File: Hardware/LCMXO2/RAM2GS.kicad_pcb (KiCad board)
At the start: 4 copper layers, 67.3 x 48.5 mm, 64 parts, among them J1 IIgs RAM Exp., J2 JTAG, U1 LCMXO2-TG100, U10 74LVC1G04GW, U11 AP2127K-1.2TRG1, U2 W9812G6KH-6, U3 60M, U4 74AHCT245PW, U5 74LVC245APW, U6 74LVC245APW, U7 74LVC245APW, U8 AZ1117CH-3.3TRG1, U9 74LVC1G04GW

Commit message: Updated LCMXO2 board, fixed GND via
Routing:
- net GND: vias 211 -> 212
- net (no net): vias 1 -> 0
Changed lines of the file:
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@@
     (add_net "Net-(U9-Pad1)")
+  )
+  (module stdpads:R_0603 (layer F.Cu)
+    (at 75.6 119.65)
+    (tags resistor)
+    (solder_mask_margin 0.05)
+    (solder_paste_margin -0.05)
+    (attr smd)
+    (fp_text reference R8 (at 0 0) (layer F.Fab)
+      (effects (font (size 0.254 0.254) (thickness 0.0635)))
+    )
+    (fp_text value 10k (at 0 0.25) (layer F.Fab)
+      (effects (font (size 0.127 0.127) (thickness 0.03175)))
+    )
+    (fp_line (start -0.8 0.4) (end -0.8 -0.4) (layer F.Fab) (width 0.1))
+    (fp_line (start -0.8 -0.4) (end 0.8 -0.4) (layer F.Fab) (width 0.1))
+    (fp_line (start 0.8 -0.4) (end 0.8 0.4) (layer F.Fab) (width 0.1))
+    (fp_line (start 0.8 0.4) (end -0.8 0.4) (layer F.Fab) (width 0.1))
+    (fp_line (start -0.162779 -0.51) (end 0.162779 -0.51) (layer F.SilkS) (width 0.12))
+    (fp_line (start -0.162779 0.51) (end 0.162779 0.51) (layer F.SilkS) (width 0.12))
+    (fp_line (start -1.4 0.7) (end -1.4 -0.7) (layer F.CrtYd) (width 0.05))
+    (fp_line (start -1.4 -0.7) (end 1.4 -0.7) (layer F.CrtYd) (width 0.05))
+    (fp_line (start 1.4 -0.7) (end 1.4 0.7) (layer F.CrtYd) (width 0.05))
+    (fp_line (start 1.4 0.7) (end -1.4 0.7) (layer F.CrtYd) (width 0.05))
+    (fp_text user %R (at 0 0) (layer F.SilkS) hide
+      (effects (font (size 0.254 0.254) (thickness 0.0635)))
+    )
+    (pad 1 smd roundrect (at -0.8 0) (size 0.7 0.95) (layers F.Cu F.Paste F.Mask) (roundrect_rratio 0.25)
+      (net 37 +3V3))
+    (pad 2 smd roundrect (at 0.8 0) (size 0.7 0.95) (layers F.Cu F.Paste F.Mask) (roundrect_rratio 0.25)
+      (net 122 /DONE))
+    (model ${KISYS3DMOD}/Resistor_SMD.3dshapes/R_0603_1608Metric.wrl
+      (at (xyz 0 0 0))
+      (scale (xyz 1 1 1))
+      (rotate (xyz 0 0 0))
+    )
   )
   (module stdpads:TSSOP-20_4.4x6.5mm_P0.65mm (layer F.Cu)
@@
       (rotate (xyz 0 0 0))
     )
-  )
-  (module stdpads:R_0603 (layer F.Cu)
-    (at 75.6 119.65)
-    (tags resistor)
-    (solder_mask_margin 0.05)
-    (solder_paste_margin -0.05)
-    (attr smd)
-    (fp_text reference R8 (at 0 0) (layer F.Fab)
-      (effects (font (size 0.254 0.254) (thickness 0.0635)))
-    )
-    (fp_text value 10k (at 0 0.25) (layer F.Fab)
-      (effects (font (size 0.127 0.127) (thickness 0.03175)))
-    )
-    (fp_line (start 1.4 0.7) (end -1.4 0.7) (layer F.CrtYd) (width 0.05))
-    (fp_line (start 1.4 -0.7) (end 1.4 0.7) (layer F.CrtYd) (width 0.05))
-    (fp_line (start -1.4 -0.7) (end 1.4 -0.7) (layer F.CrtYd) (width 0.05))
-    (fp_line (start -1.4 0.7) (end -1.4 -0.7) (layer F.CrtYd) (width 0.05))
-    (fp_line (start -0.162779 0.51) (end 0.162779 0.51) (layer F.SilkS) (width 0.12))
-    (fp_line (start -0.162779 -0.51) (end 0.162779 -0.51) (layer F.SilkS) (width 0.12))
-    (fp_line (start 0.8 0.4) (end -0.8 0.4) (layer F.Fab) (width 0.1))
-    (fp_line (start 0.8 -0.4) (end 0.8 0.4) (layer F.Fab) (width 0.1))
-    (fp_line (start -0.8 -0.4) (end 0.8 -0.4) (layer F.Fab) (width 0.1))
-    (fp_line (start -0.8 0.4) (end -0.8 -0.4) (layer F.Fab) (width 0.1))
-    (fp_text user %R (at 0 0) (layer F.SilkS) hide
-      (effects (font (size 0.254 0.254) (thickness 0.0635)))
-    )
-    (pad 2 smd roundrect (at 0.8 0) (size 0.7 0.95) (layers F.Cu F.Paste F.Mask) (roundrect_rratio 0.25)
-      (net 122 /DONE))
-    (pad 1 smd roundrect (at -0.8 0) (size 0.7 0.95) (layers F.Cu F.Paste F.Mask) (roundrect_rratio 0.25)
-      (net 37 +3V3))
   )
   (module stdpads:LED_0805 (layer F.Cu)
@@
     (pad 1 smd roundrect (at -0.75 0 270) (size 0.85 0.95) (layers F.Cu F.Paste F.Mask) (roundrect_rratio 0.25)
       (net 37 +3V3))
-    (model ${KISYS3DMOD}/Capacitor_SMD.3dshapes/C_0603_1608Metric.wrl
-      (at (xyz 0 0 0))
-      (scale (xyz 1 1 1))
-      (rotate (xyz 0 0 0))
-    )
   )
   (module stdpads:Fiducial (layer F.Cu)
@@
   (gr_line (start 55.372 139.192) (end 55.372 132.08) (layer Edge.Cuts) (width 0.15))
   (gr_line (start 112.776 139.7) (end 55.88 139.7) (layer Edge.Cuts) (width 0.15))
-  (via (at 107.15 118.5) (size 0.5) (drill 0.2) (layers F.Cu B.Cu) (net 0) (status 40000))
+  (via (at 107.15 118.5) (size 0.5) (drill 0.2) (layers F.Cu B.Cu) (net 1) (status 40000))
   (via (at 85.471 94.996) (size 0.5) (drill 0.2) (layers F.Cu B.Cu) (net 1))
   (via (at 80.391 94.742) (size 0.5) (drill 0.2) (layers F.Cu B.Cu) (net 1))

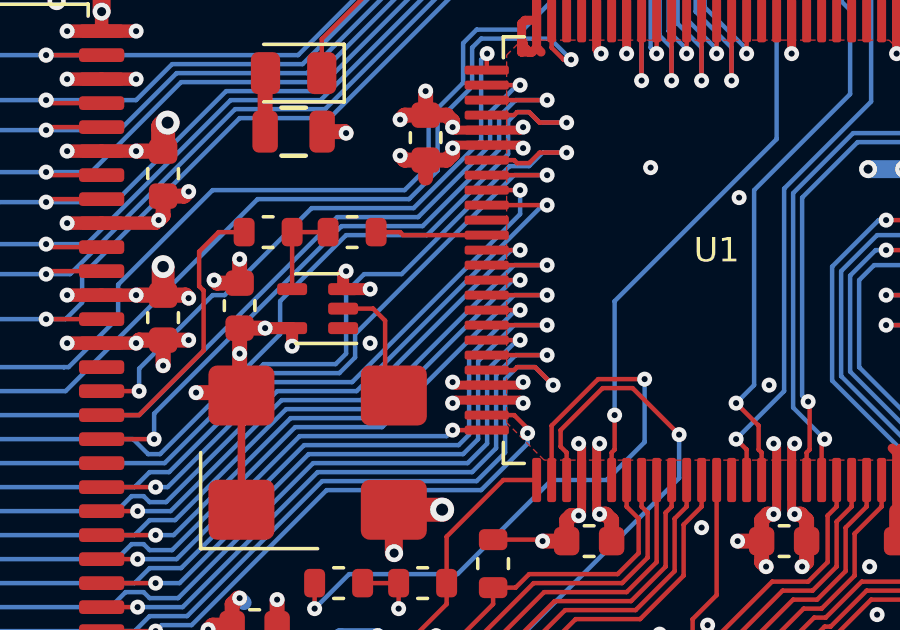
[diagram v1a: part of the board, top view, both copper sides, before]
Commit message: Documentation update
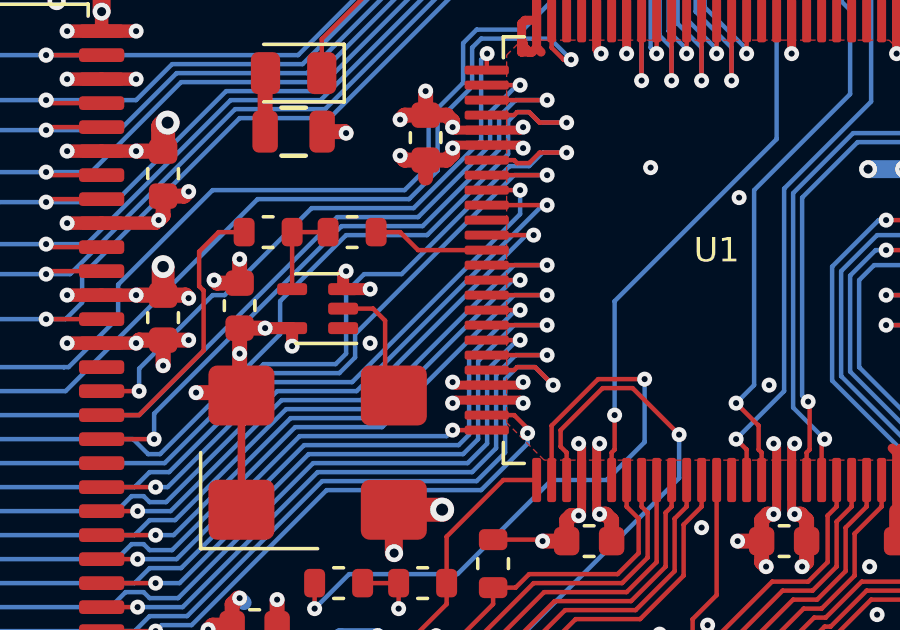
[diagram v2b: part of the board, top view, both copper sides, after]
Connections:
- U1 pad 62: /AClk -> /RA9
- U1 pad 63: /RA9 -> /AClk
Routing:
- net /RA9: track 18.7 -> 19.8 mm
